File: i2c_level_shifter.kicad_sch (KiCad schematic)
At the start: 0 parts

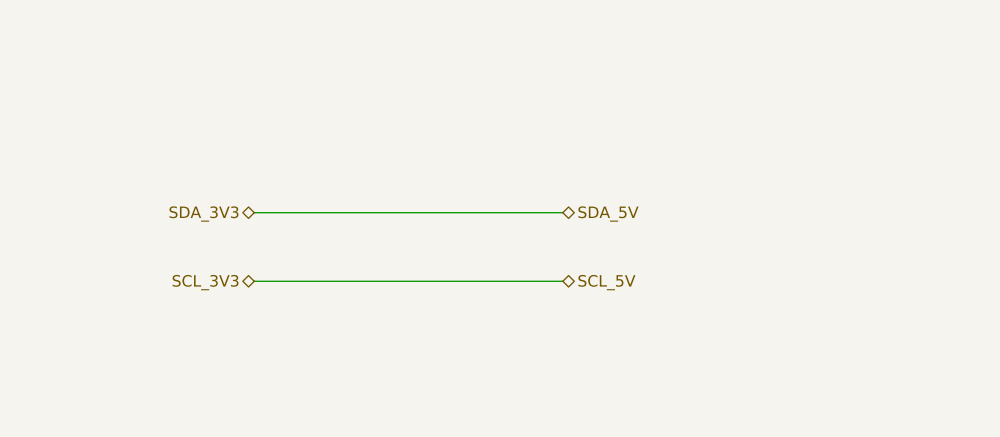
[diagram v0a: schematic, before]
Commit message: 2/26 Work as a team
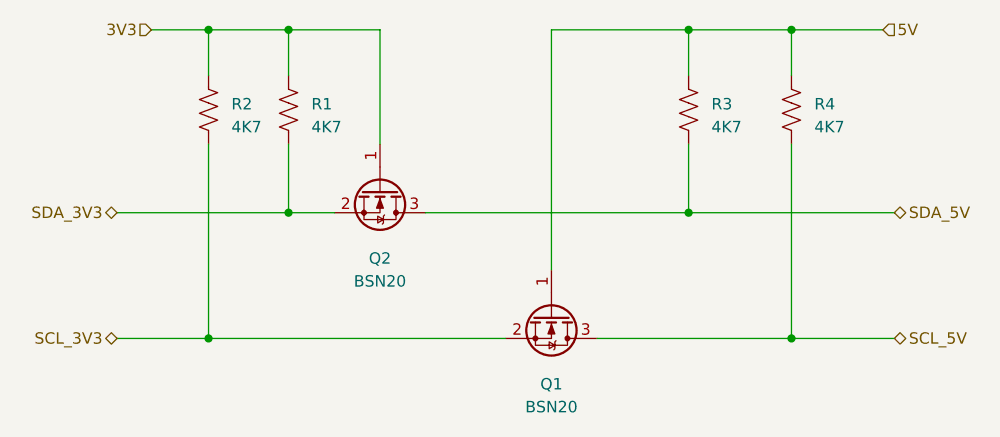
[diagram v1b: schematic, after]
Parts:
- added Q1, Q2: BSN20, Package_TO_SOT_SMD:SOT-23, symbol Transistor_FET:BSN20
- added R1, R2, R3, R4: 4K7, symbol Device:R_US
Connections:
- net SCL_3V3: now also Q1.2 (S), R2.2
- net SDA_3V3: now also Q2.2 (S), R1.2
- new net 3V3: Q2.1 (G), R1.1, R2.1
- new net 5V: Q1.1 (G), R3.1, R4.1
- new net SCL_5V: Q1.3 (D), R4.2
- new net SDA_5V: Q2.3 (D), R3.2
